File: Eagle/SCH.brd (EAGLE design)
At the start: 81.3 x 46.7 mm, 28 parts, among them IC1 L7805, IC2 L7805, Q1 IRF540, Q2 IRF540, Q3 IRF540, U1 ARDUINO-NANO

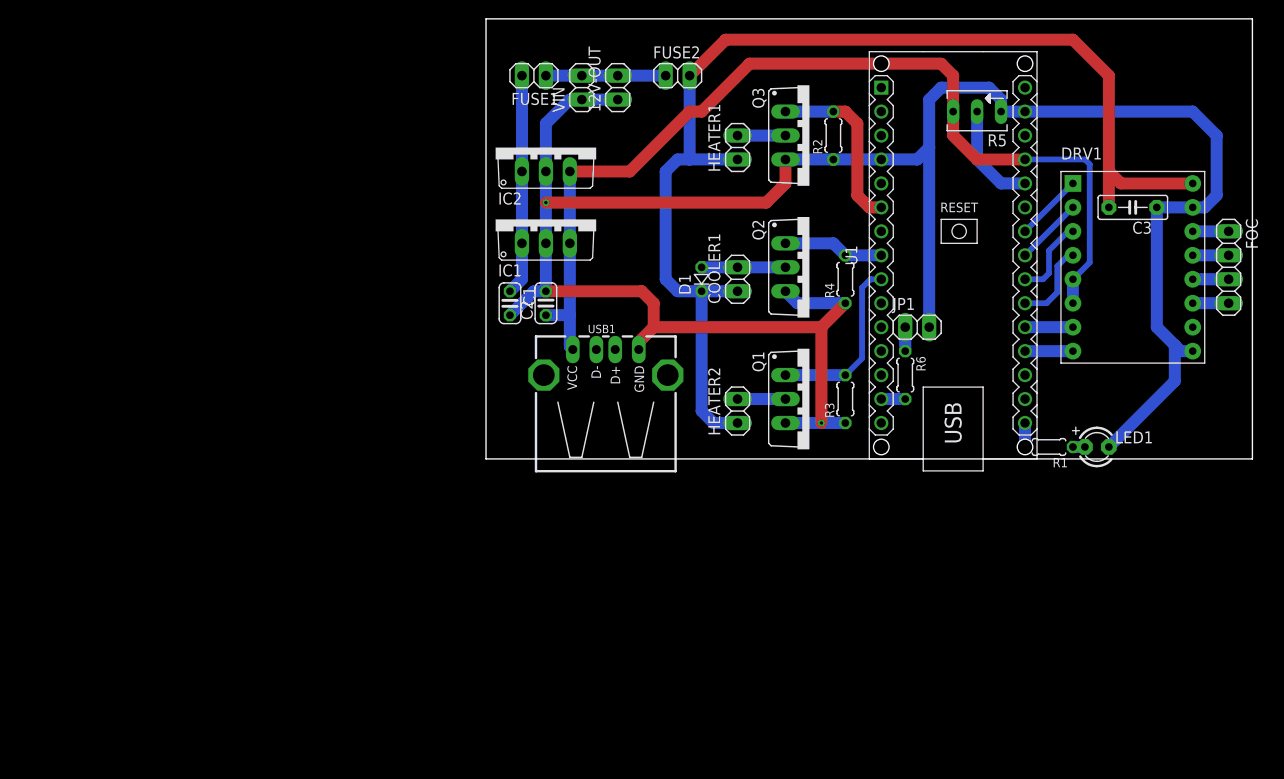
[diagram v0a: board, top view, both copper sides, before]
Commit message: New PCB design
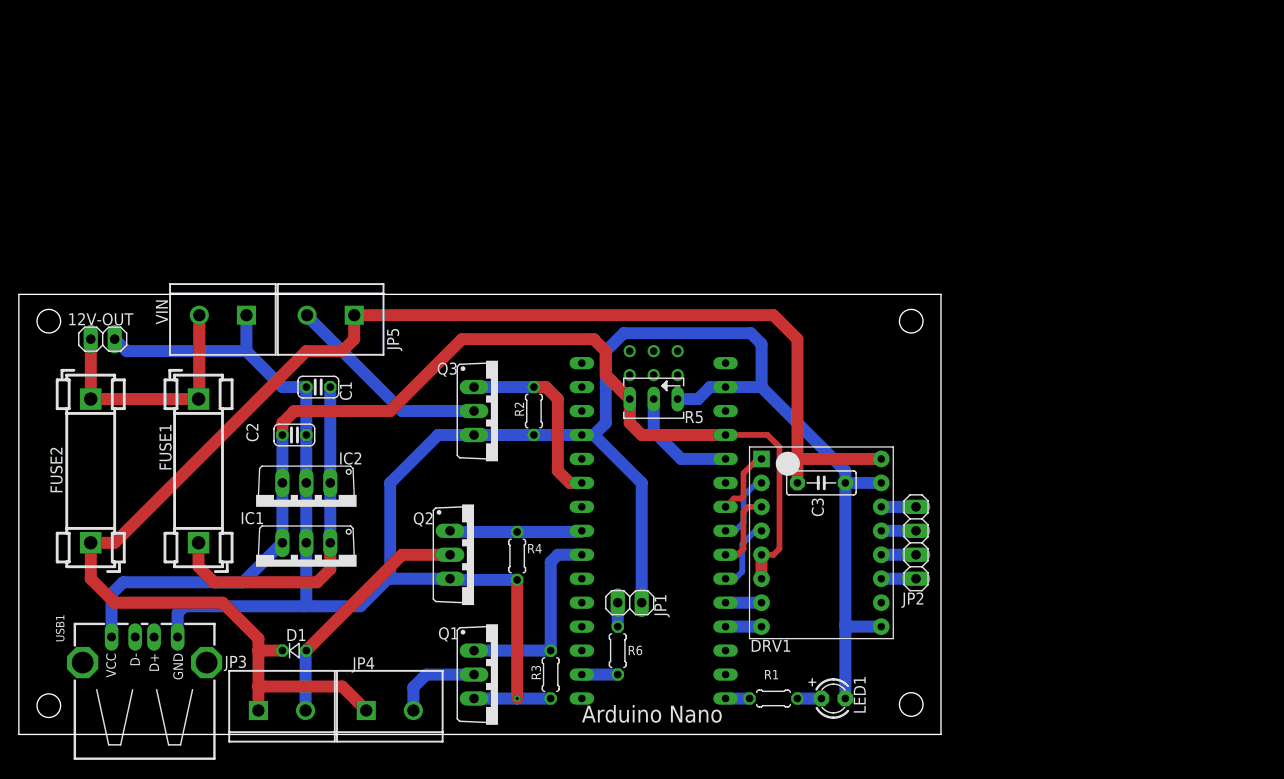
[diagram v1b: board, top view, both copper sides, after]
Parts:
- removed COOLER1, HEATER1, HEATER2: (no value), pinhead:1X02
- removed FOC: (no value), pinhead:1X04
- removed U1: ARDUINO-NANO, DIY:ARDUINO-NANO-3.0
- added JP2: FOCUSER, pinhead:1X04
- added JP3, JP4, JP5: (no value), SparkFun-Connectors:SCREWTERMINAL-5MM-2
- added U$1: NANO, Arduino-clone:NANO
- FUSE1: value (none) -> 1.5A; device pinhead:1X02 -> fuse:FUSE_HOLDER_5X20MM
- FUSE2: value (none) -> 2A; device pinhead:1X02 -> fuse:FUSE_HOLDER_5X20MM
- VIN: device pinhead:1X02 -> SparkFun-Connectors:SCREWTERMINAL-5MM-2
- moved FUSE2 71.1 mm to (-41.9, 6.35), turned to 270 degrees
- moved 12V-OUT 60.8 mm to (-40.6, 12.7), turned to 180 degrees
- moved D1 58.4 mm to (-20.3, -20.3), turned to 0 degrees
- moved USB1 57.6 mm to (-36.2, -21.6)
- moved FUSE1 49.4 mm to (-30.5, 6.35), turned to 270 degrees
- moved Q2 46.8 mm to (-1.27, -10.2)
- moved R5 45.9 mm to (17.8, 6.35)
- moved IC2 45.8 mm to (-19.1, -5.08), turned to 180 degrees
- moved R4 45.5 mm to (3.30, -10.3)
- moved IC1 44.7 mm to (-19.1, -11.4), turned to 180 degrees
- moved C3 44.1 mm to (35.6, -2.54)
- moved DRV1 44.1 mm to (27.9, 1.27)
- moved Q1 44.1 mm to (1.27, -22.9)
- moved Q3 44.1 mm to (1.27, 5.08)
- moved R2 43.1 mm to (5.08, 5.08)
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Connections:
- removed net 3V3: U1.J2.14
- removed net VIN: U1.J2.1
- net +12V: now also JP3.1, JP4.1, JP5.1; no longer COOLER1.1, HEATER1.1, HEATER2.1
- net +5V: now also U$1.5V; no longer U1.J2.4
- net D13: now also U$1.D13; no longer U1.J2.15
- net D3: now also U$1.D3; no longer U1.J1.6
- net D5: now also U$1.D5; no longer U1.J1.8
- net D6: now also U$1.D6; no longer U1.J1.9
- net GND: now also U$1.GND, U$1.GND1; no longer U1.J1.4, U1.J2.2
- net N$10: now also JP4.2; no longer HEATER2.2
- net N$11: now also JP5.2; no longer HEATER1.2
- net N$12: now also U$1.A1; no longer U1.J2.11
- net N$13: now also JP2.1; no longer FOC.1
- net N$14: now also JP2.2; no longer FOC.2
- net N$15: now also JP2.3; no longer FOC.3
- net N$16: now also JP2.4; no longer FOC.4
- net N$17: now also U$1.A2; no longer U1.J2.10
- net N$18: now also U$1.A3; no longer U1.J2.9
- net N$2: now also U$1.A7; no longer U1.J2.5
- net N$20: now also U$1.A4; no longer U1.J2.8
- net N$3: now also U$1.D11; no longer U1.J1.14
- net N$5: now also U$1.A0; no longer U1.J2.12
- net N$6: now also U$1.A5; no longer U1.J2.7
- net N$9: now also JP3.2; no longer COOLER1.2
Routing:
- net +12V: track 124.6 -> 158.6 mm
- net N$9: track 8.89 -> 25.8 mm
- net N$11: track 5.08 -> 22.0 mm
- net N$8: track 12.7 -> 26.7 mm
- net N$4: track 23.4 -> 37.1 mm
- net +5V: track 105.0 -> 117.2 mm
- net GND: track 240.6 -> 249.8 mm, vias 2 -> 1
- net N$10: track 5.08 -> 9.45 mm
- net D5: track 10.7 -> 14.1 mm
- net D6: track 18.8 -> 21.1 mm
- net D3: track 18.8 -> 20.1 mm
- net N$5: track 5.08 -> 3.81 mm
- net N$12: track 5.08 -> 3.81 mm
- net N$1: track 1.27 -> 2.54 mm
- net N$3: track 2.54 -> 3.81 mm
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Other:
- board size 81.3 x 46.7 mm -> 97.8 x 46.7 mm
- board text added: "Arduino Nano"
